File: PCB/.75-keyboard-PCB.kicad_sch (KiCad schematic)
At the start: 177 parts, among them J1 SW_Push_45deg, K1 SW_Push_45deg, M1 SW_Push_45deg, P1 SW_Push_45deg, Q1 SW_Push_45deg, T1 SW_Push_45deg, U1 SW_Push_45deg, X1 SW_Push_45deg, Y1 SW_Push_45deg

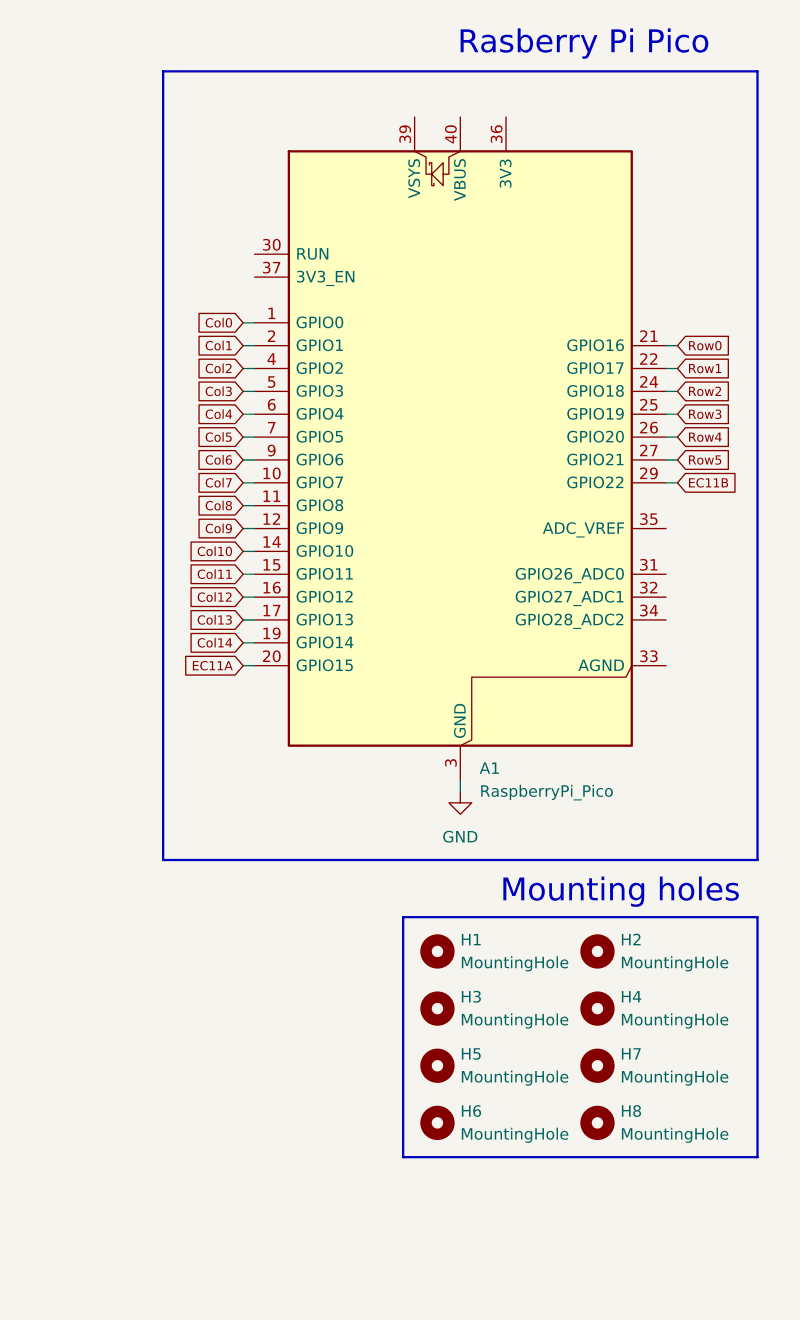
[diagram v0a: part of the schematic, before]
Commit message: pcb routing finished
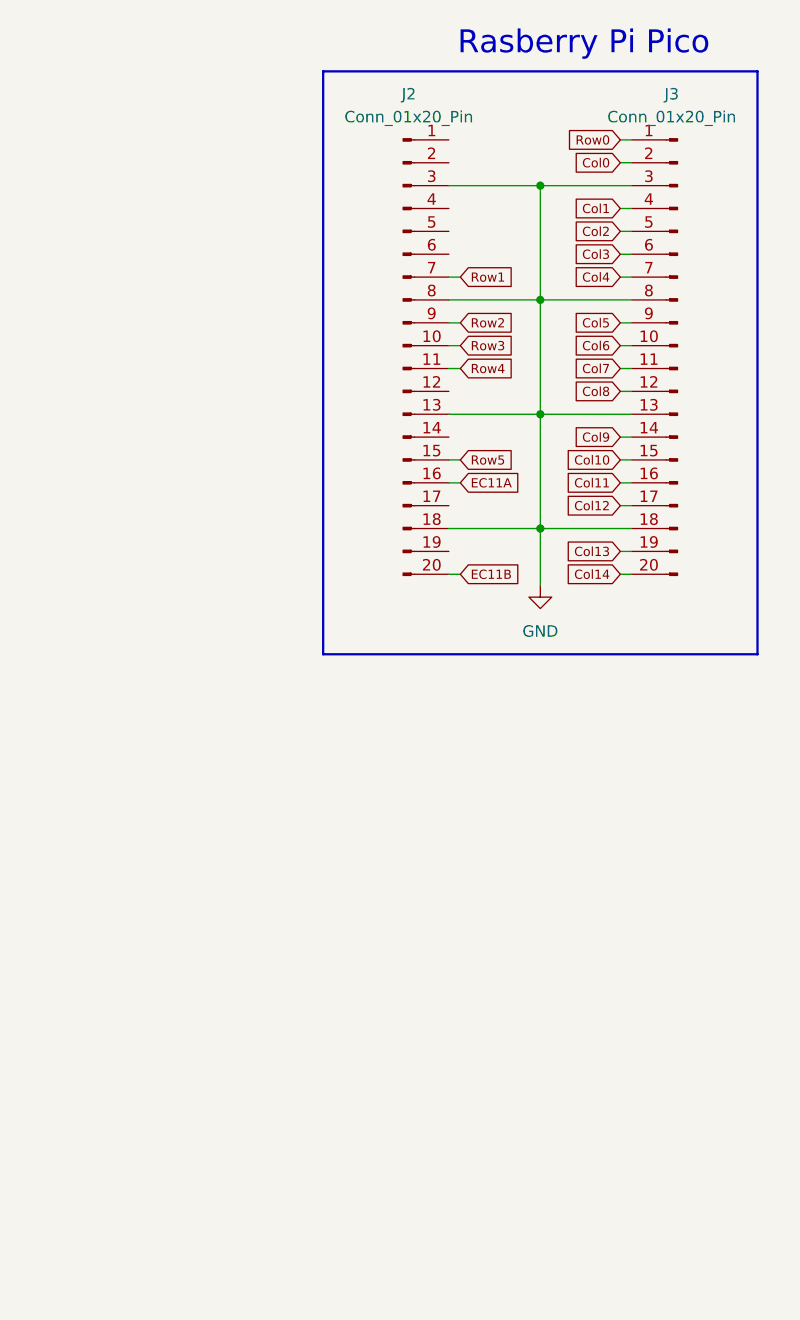
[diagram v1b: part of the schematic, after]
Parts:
- removed A1: RaspberryPi_Pico, Module:RaspberryPi_Pico_Common_Unspecified, symbol MCU_Module:RaspberryPi_Pico
- removed H1, H2, H3, H4, H5, H6, H7, H8: MountingHole, MountingHole:MountingHole_3.2mm_M3, symbol Mechanical:MountingHole
- added J2, J3: Conn_01x20_Pin, Connector_PinSocket_2.54mm:PinSocket_1x20_P2.54mm_Vertical, symbol Connector:Conn_01x20_Pin
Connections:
- net Col0: now also J3.2 (Pin_2)
- net Col1: now also J3.4 (Pin_4)
- net Col10: now also J3.15 (Pin_15)
- net Col11: now also J3.16 (Pin_16)
- net Col12: now also J3.17 (Pin_17)
- net Col13: now also J3.19 (Pin_19)
- net Col14: now also J3.20 (Pin_20)
- net Col2: now also J3.5 (Pin_5)
- net Col3: now also J3.6 (Pin_6)
- net Col4: now also J3.7 (Pin_7)
- net Col5: now also J3.9 (Pin_9)
- net Col6: now also J3.10 (Pin_10)
- net Col7: now also J3.11 (Pin_11)
- net Col8: now also J3.12 (Pin_12)
- net Col9: now also J3.14 (Pin_14)
- net EC11A: now also J2.16 (Pin_16)
- net EC11B: now also J2.20 (Pin_20)
- net GND: now also J2.13 (Pin_13), J2.18 (Pin_18), J2.3 (Pin_3), J2.8 (Pin_8), J3.13 (Pin_13), J3.18 (Pin_18), J3.3 (Pin_3), J3.8 (Pin_8)
- net Row0: now also J3.1 (Pin_1)
- net Row1: now also J2.7 (Pin_7)
- net Row2: now also J2.9 (Pin_9)
- net Row3: now also J2.10 (Pin_10)
- net Row4: now also J2.11 (Pin_11)
- net Row5: now also J2.15 (Pin_15)
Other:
- note removed: "Mounting holes"

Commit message: kicad switch models
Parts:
- '1, ,1, -1, .1, /1, ;1, <1, =1, >1, A2, Alt2, B1, C1, Ctrl2, D30, Del1, E1, End1, Esc1, F1, F10, F11, F12, F13, F2, F3, F4, F5, F6, F7, F8, F9, Fn1, G1, H9, Home1, I1, Insert1, J1, K1, L1, M1, N10, O1, P1, PgDn1, PgUp1, Q1, R1, S1, T1, U1, V1, V2, W1, X1, Y1, Z1, [1, ]1, ^1, n0, n1, n2, n3, n4, n5, n6, n7, n8, n9, ~1: footprint Button_Switch_Keyboard:SW_Cherry_MX_1.00u_PCB -> Library:3DSW_Cherry_MX_1.00u_PCB
- Alt1, Ctrl1, Win1: footprint Button_Switch_Keyboard:SW_Cherry_MX_1.25u_PCB -> Library:3DSW_Cherry_MX_1.25u_PCB
- Backspace1: footprint Button_Switch_Keyboard:SW_Cherry_MX_2.00u_PCB -> Library:3DSW_Cherry_MX_2.00u_PCB
- Caps1, Shift2: footprint Button_Switch_Keyboard:SW_Cherry_MX_1.75u_PCB -> Library:3D_SW_Cherry_MX_1.75u_PCB
- Enter1, Shift1: footprint Button_Switch_Keyboard:SW_Cherry_MX_2.25u_PCB -> Library:3DSW_Cherry_MX_2.25u_PCB
- Space1: footprint Button_Switch_Keyboard:SW_Cherry_MX_6.25u_PCB -> Library:3DSW_Cherry_MX_6.25u_PCB
- Tab1, \1: footprint Button_Switch_Keyboard:SW_Cherry_MX_1.50u_PCB -> Library:3DSW_Cherry_MX_1.50u_PCB
